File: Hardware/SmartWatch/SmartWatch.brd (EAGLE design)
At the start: 36.8 x 36.8 mm, 36 parts, among them U1 STM32L476, U3 UG-2828GDEDF11, U4 FAN5331SX, U5 APDS-9960

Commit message: renamed part
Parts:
- renumbered U$27 to U6
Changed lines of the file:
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@@
 <element name="C12" library="resistor" package="C1206" value="47uF" x="5.08" y="2.54"/>
 <element name="C1" library="microbuilder" package="0603-MINI" value="1uF" x="33.02" y="11.43" rot="R90"/>
-<element name="U$27" library="SmartWatch" package="28QFN4X4" value="LTC3557" x="17.78" y="15.24"/>
+<element name="U6" library="SmartWatch" package="28QFN4X4" value="LTC3557" x="17.78" y="15.24"/>
 </elements>
 <signals>

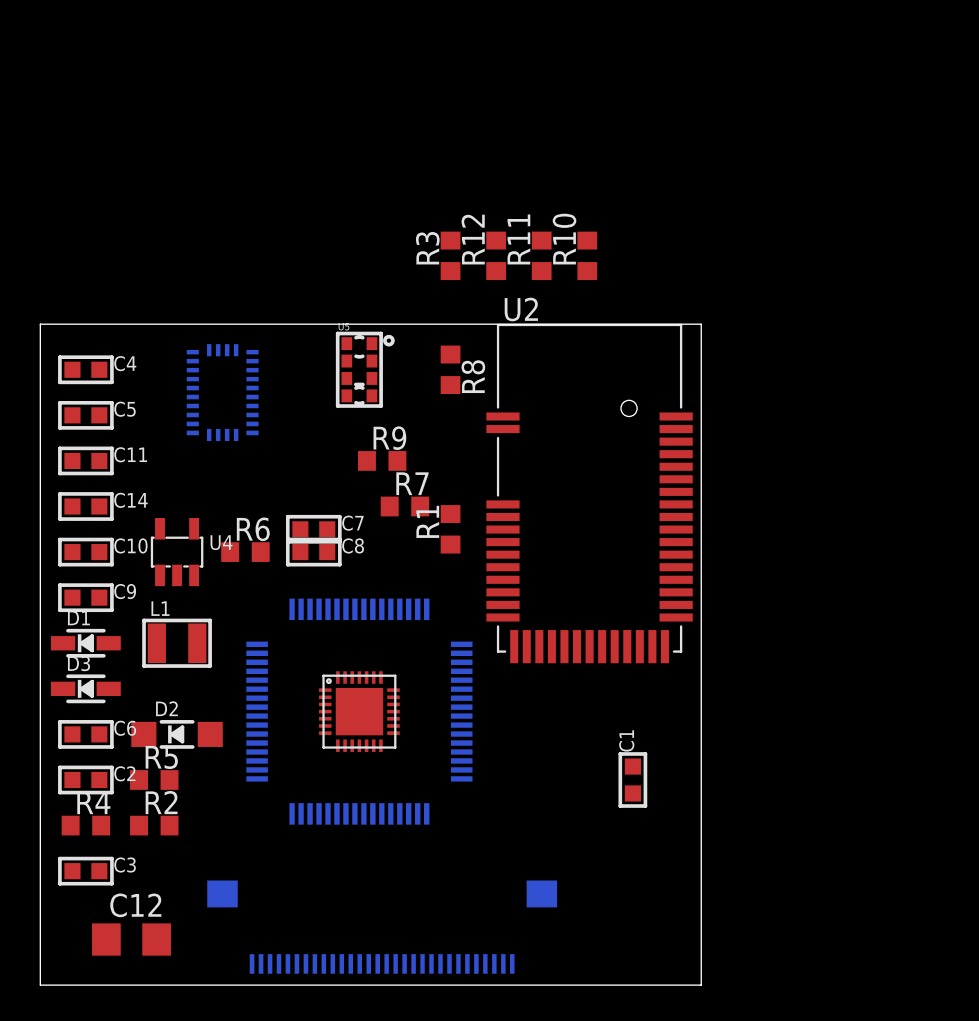
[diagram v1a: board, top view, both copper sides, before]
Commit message: Updated schematic
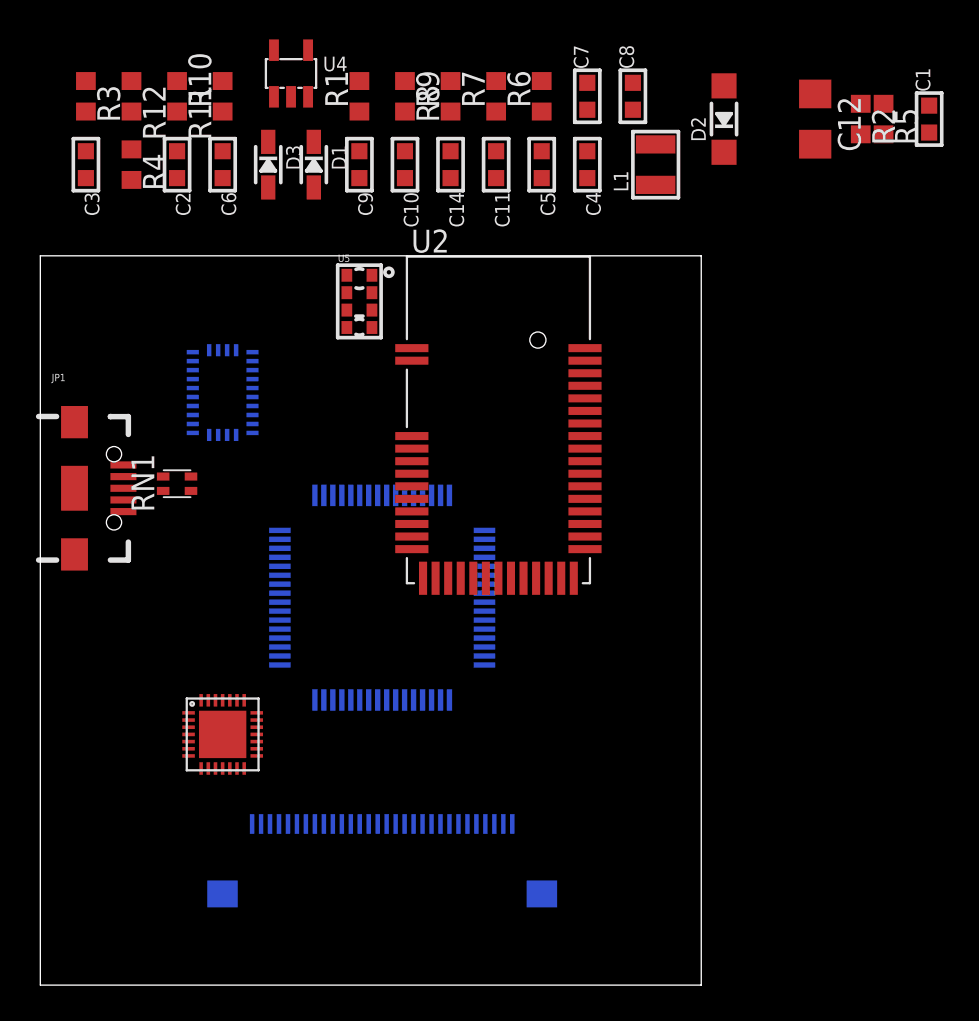
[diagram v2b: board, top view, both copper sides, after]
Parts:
- added JP1: (no value), SparkFun-Connectors:USB-B-MICRO-SMD_V03
- added RN1: (no value), MicroBoard:EXBV4V
- moved C12 59.5 mm to (43.2, 48.3), turned to 270 degrees
- moved R2 55.7 mm to (45.7, 48.3), turned to 270 degrees
- moved R5 54.8 mm to (47.0, 48.3), turned to 270 degrees
- moved D2 45.9 mm to (38.1, 48.3), turned to 90 degrees
- moved C1 40.4 mm to (49.5, 48.3)
- moved C3 39.4 mm to (2.54, 45.7), turned to 270 degrees
- moved L1 37.7 mm to (34.3, 45.7), turned to 90 degrees
- moved R4 36.9 mm to (5.08, 45.7), turned to 270 degrees
- moved C2 34.7 mm to (7.62, 45.7), turned to 270 degrees
- moved C6 32.7 mm to (10.2, 45.7), turned to 270 degrees
- moved C8 31.0 mm to (33.0, 49.5), turned to 90 degrees
- moved D3 30.9 mm to (12.7, 45.7), turned to 270 degrees
- moved R6 30.3 mm to (27.9, 49.5), turned to 90 degrees
- moved C4 30.2 mm to (30.5, 45.7), turned to 270 degrees
- moved D1 29.5 mm to (15.2, 45.7), turned to 270 degrees
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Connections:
- new net D+: RN1.4
- new net D-: RN1.3
- new net N$10: JP1.D+1, RN1.1
- new net N$15: JP1.D-1, RN1.2
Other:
- board size 36.8 x 36.8 mm -> 36.8 x 40.6 mm
